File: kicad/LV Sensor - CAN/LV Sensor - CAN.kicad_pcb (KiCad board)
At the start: 2 copper layers, 26.2 x 30 mm, 9 parts, among them J2 Conn_01x09_Pin, U1 MCP2518FD-xJHA, U2 DSC1001DL5-020.0000T, U5 ATA6561-GAQW-N

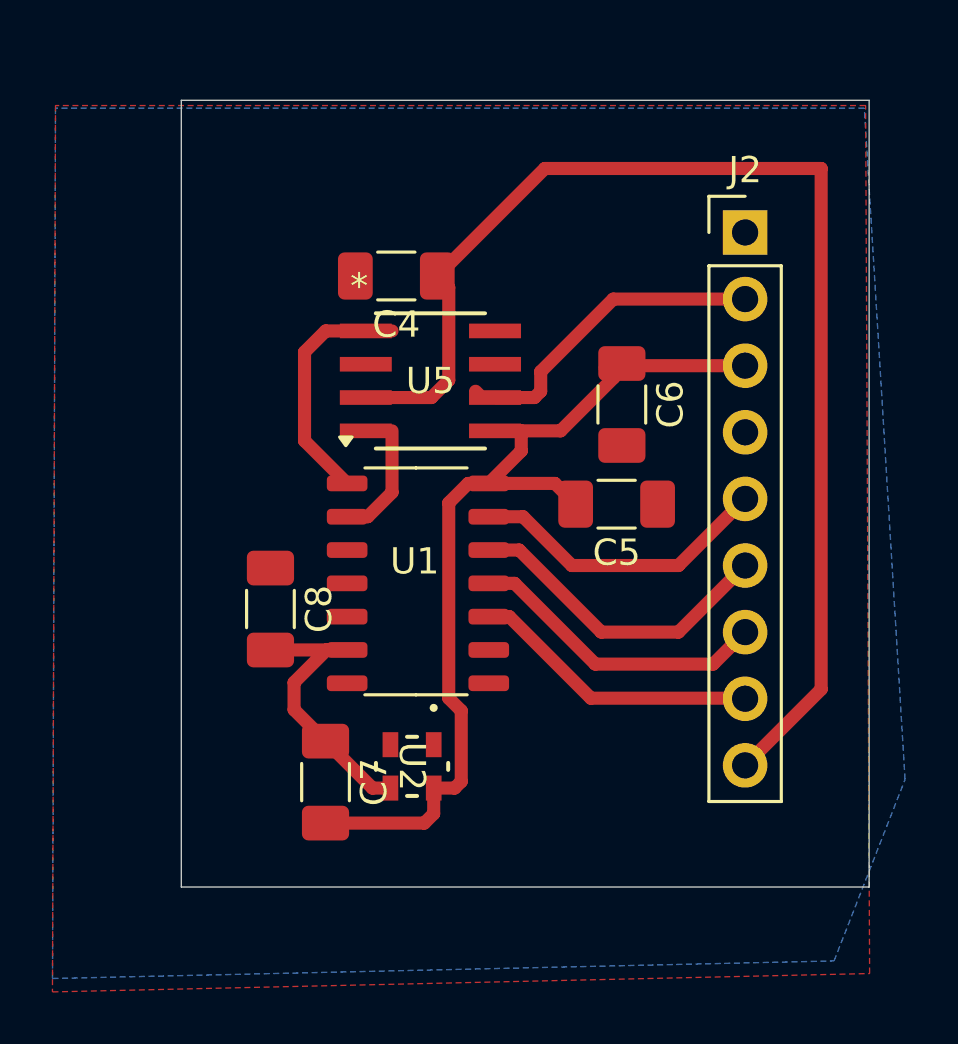
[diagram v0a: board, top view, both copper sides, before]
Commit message: 09-10-25
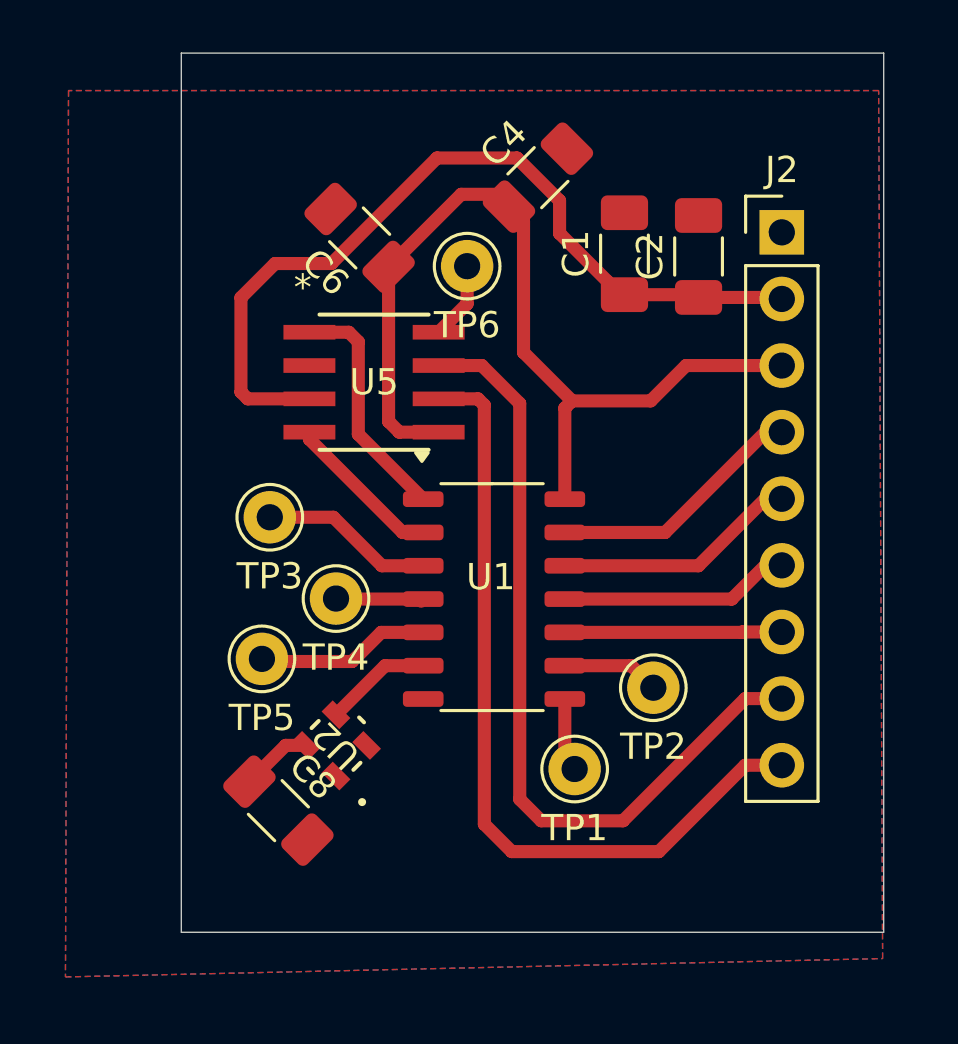
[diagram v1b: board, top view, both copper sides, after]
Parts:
- removed C5: 0.1uF, Capacitor_SMD:C_1206_3216Metric_Pad1.33x1.80mm_HandSolder
- removed C7: 0.01uF, Capacitor_SMD:C_1206_3216Metric_Pad1.33x1.80mm_HandSolder
- added C1: 100nF, Capacitor_SMD:C_1206_3216Metric_Pad1.33x1.80mm_HandSolder, F.Cu at (122.6, 36.2)
- added C2: 100nF, Capacitor_SMD:C_1206_3216Metric_Pad1.33x1.80mm_HandSolder, F.Cu at (125.4, 36.4)
- added TP1: TestPoint, Connector_Pin:Pin_D1.0mm_L10.0mm, F.Cu at (120.7, 55.9)
- added TP2: TestPoint, Connector_Pin:Pin_D1.0mm_L10.0mm, F.Cu at (123.7, 52.8)
- added TP3: TestPoint, Connector_Pin:Pin_D1.0mm_L10.0mm, F.Cu at (109.1, 46.3)
- added TP4: TestPoint, Connector_Pin:Pin_D1.0mm_L10.0mm, F.Cu at (111.6, 49.4)
- added TP5: TestPoint, Connector_Pin:Pin_D1.0mm_L10.0mm, F.Cu at (108.8, 51.7)
- added TP6: TestPoint, Connector_Pin:Pin_D1.0mm_L10.0mm, F.Cu at (116.6, 36.7)
- moved C6 11.8 mm to (112.5, 35.6), turned to 135 degrees
- moved C8 7.69 mm to (109.4, 57.5), turned to -45 degrees
- moved C4 6.57 mm to (119.3, 33.4), turned to 45 degrees
- moved U2 3.01 mm to (111.6, 55.0), turned to 135 degrees
- moved U1 2.96 mm to (117.5, 49.4)
- moved U5 2.15 mm to (113.0, 41.1)
- moved J2 1.40 mm to (128.6, 35.4)
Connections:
- net /RXCAN renamed Net-(U1-RXCAN)
- net /TXCAN renamed Net-(U1-TXCAN)
- C4 pad 1: +5V -> +3.3V
- C8 pad 1: GND -> +3V3
- C8 pad 2: Net-(U1-OSC1) -> GND
- J2 pad 1: /CANH -> GND
- J2 pad 2: /CANL -> +5V
- J2 pad 4: GND -> Net-(J2-Pin_4)
- J2 pad 5: /CS -> Net-(J2-Pin_5)
- J2 pad 6: /SDO -> Net-(J2-Pin_6)
- J2 pad 7: /SDIO -> Net-(J2-Pin_7)
- J2 pad 8: /SCK -> /CAN_H
- J2 pad 9: +5V -> /CAN_L
- U1 pad 10: /SCK -> Net-(J2-Pin_7)
- U1 pad 11: /SDIO -> Net-(J2-Pin_6)
- U1 pad 12: /SDO -> Net-(J2-Pin_5)
- U1 pad 13: /CS -> Net-(J2-Pin_4)
- U1 pad 3: GND -> Net-(U1-CLKO/SOF)
- U1 pad 4: unconnected-(U1-~{INT}-Pad4) -> Net-(U1-~{INT})
- U1 pad 5: GND -> Net-(U1-OSC2)
- U1 pad 8: unconnected-(U1-~{INT1}/GPIO1-Pad8) -> Net-(U1-~{INT1}/GPIO1)
- U1 pad 9: unconnected-(U1-~{INT0}/GPIO0/XSTBY-Pad9) -> Net-(U1-~{INT0}/GPIO0/XSTBY)
- U2 pad 4: +3.3V -> +3V3
- U5 pad 6: /CANL -> /CAN_L
- U5 pad 7: /CANH -> /CAN_H
- U5 pad 8: GND -> Net-(U5-STBY)
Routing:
- net /CAN_H: track 0.00 -> 31.0 mm
- net /CAN_L: track 0.00 -> 31.0 mm
- net +5V: track 46.9 -> 31.8 mm
- net /CANL: track 13.4 -> 0.00 mm
- net /SDO: track 12.1 -> 0.00 mm
- net /CS: track 11.6 -> 0.00 mm
- net /SDIO: track 11.6 -> 0.00 mm
- net /SCK: track 11.1 -> 0.00 mm
- net Net-(J2-Pin_4): track 0.00 -> 9.86 mm
- net Net-(J2-Pin_5): track 0.00 -> 9.33 mm
- net Net-(J2-Pin_6): track 0.00 -> 8.81 mm
- net Net-(J2-Pin_7): track 0.00 -> 8.31 mm
- net Net-(U1-OSC1): track 11.4 -> 4.10 mm
- net Net-(U1-CLKO/SOF): track 0.00 -> 6.62 mm
- net Net-(U1-OSC2): track 0.00 -> 6.01 mm
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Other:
- board size 26.2 x 30 mm -> 26.8 x 33.5 mm

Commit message: ljklj
Changed notation 3V3 to 3.3V

Co-Authored-By: Manish Shrestha <manish.shr006@gmail.com>
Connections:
- C8 pad 1: +3V3 -> +3.3V
- U2 pad 4: +3V3 -> +3.3V
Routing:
- net +3.3V: track 34.7 -> 37.4 mm
- net +3V3: track 2.71 -> 0.00 mm
